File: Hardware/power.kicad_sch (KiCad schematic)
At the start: 52 parts, among them J1 USB4110GFA, Q1 AO3407A, U1 TPS54302, U2 USBLC6-2SC6, U3 INA226, U4 AP63205WU, U5 AP2112K-3.3, U6 AP7343-33W5-7

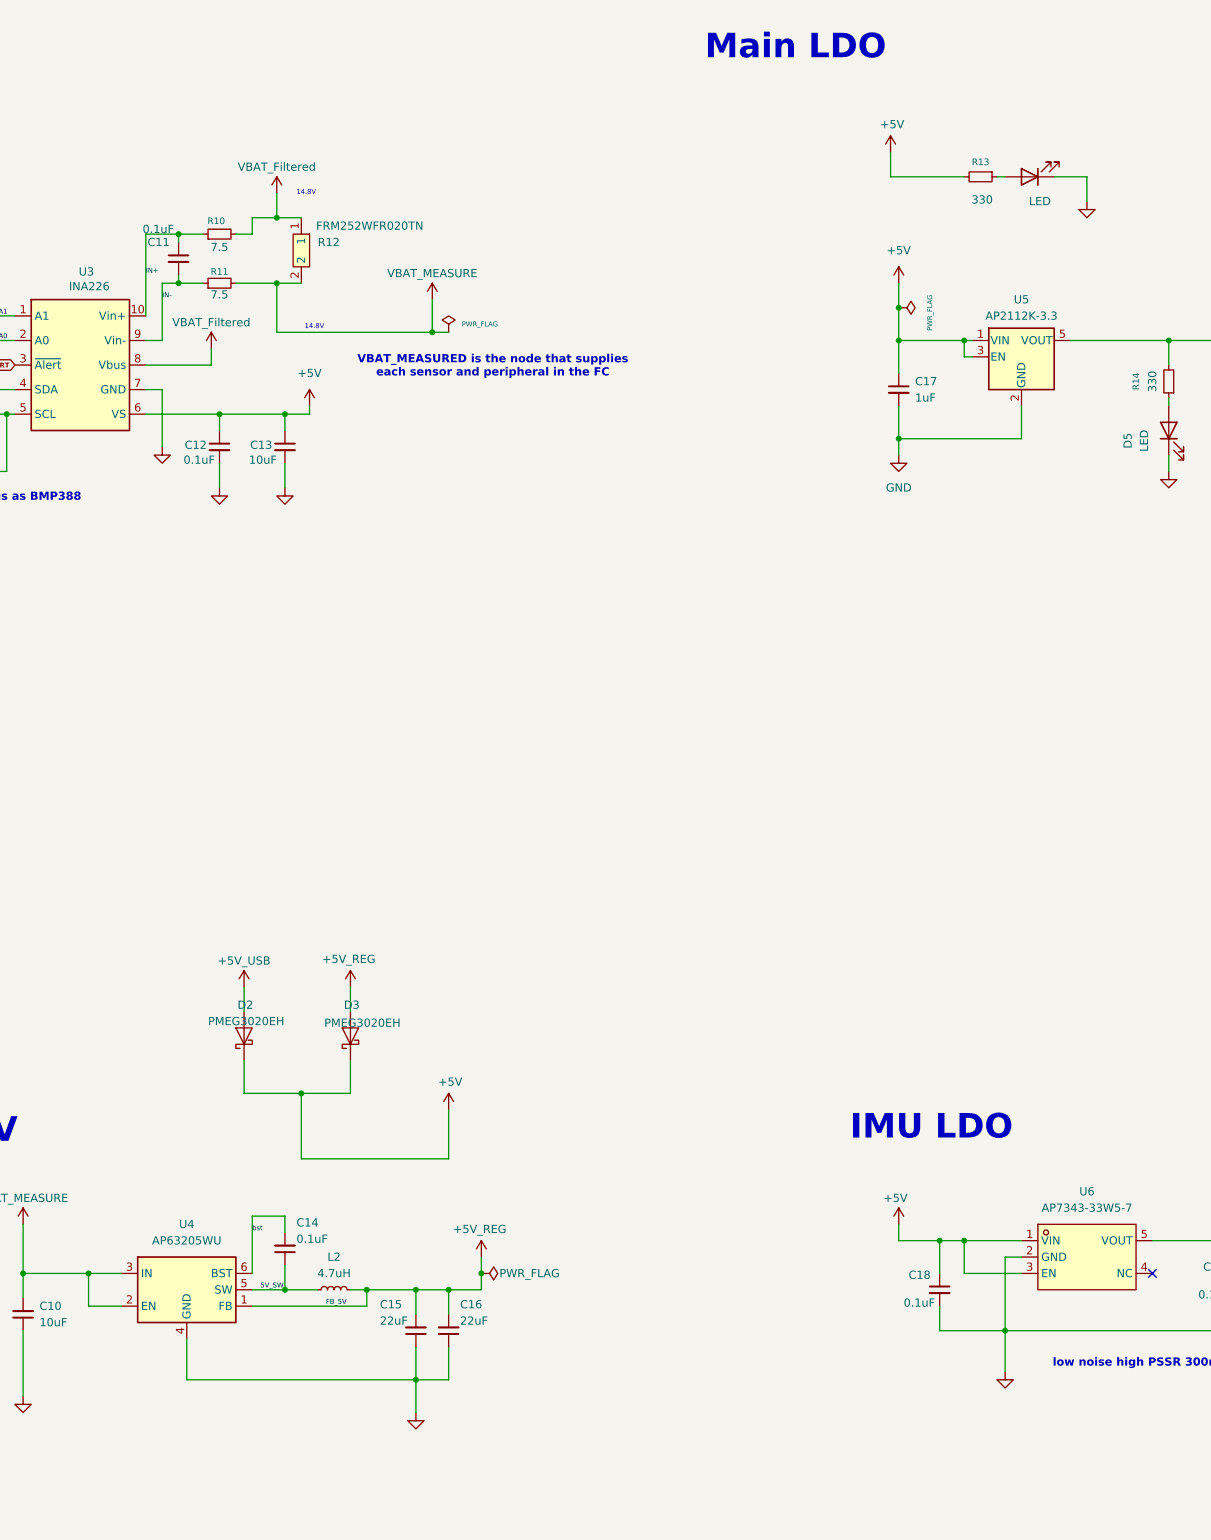
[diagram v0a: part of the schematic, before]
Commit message: progress layout
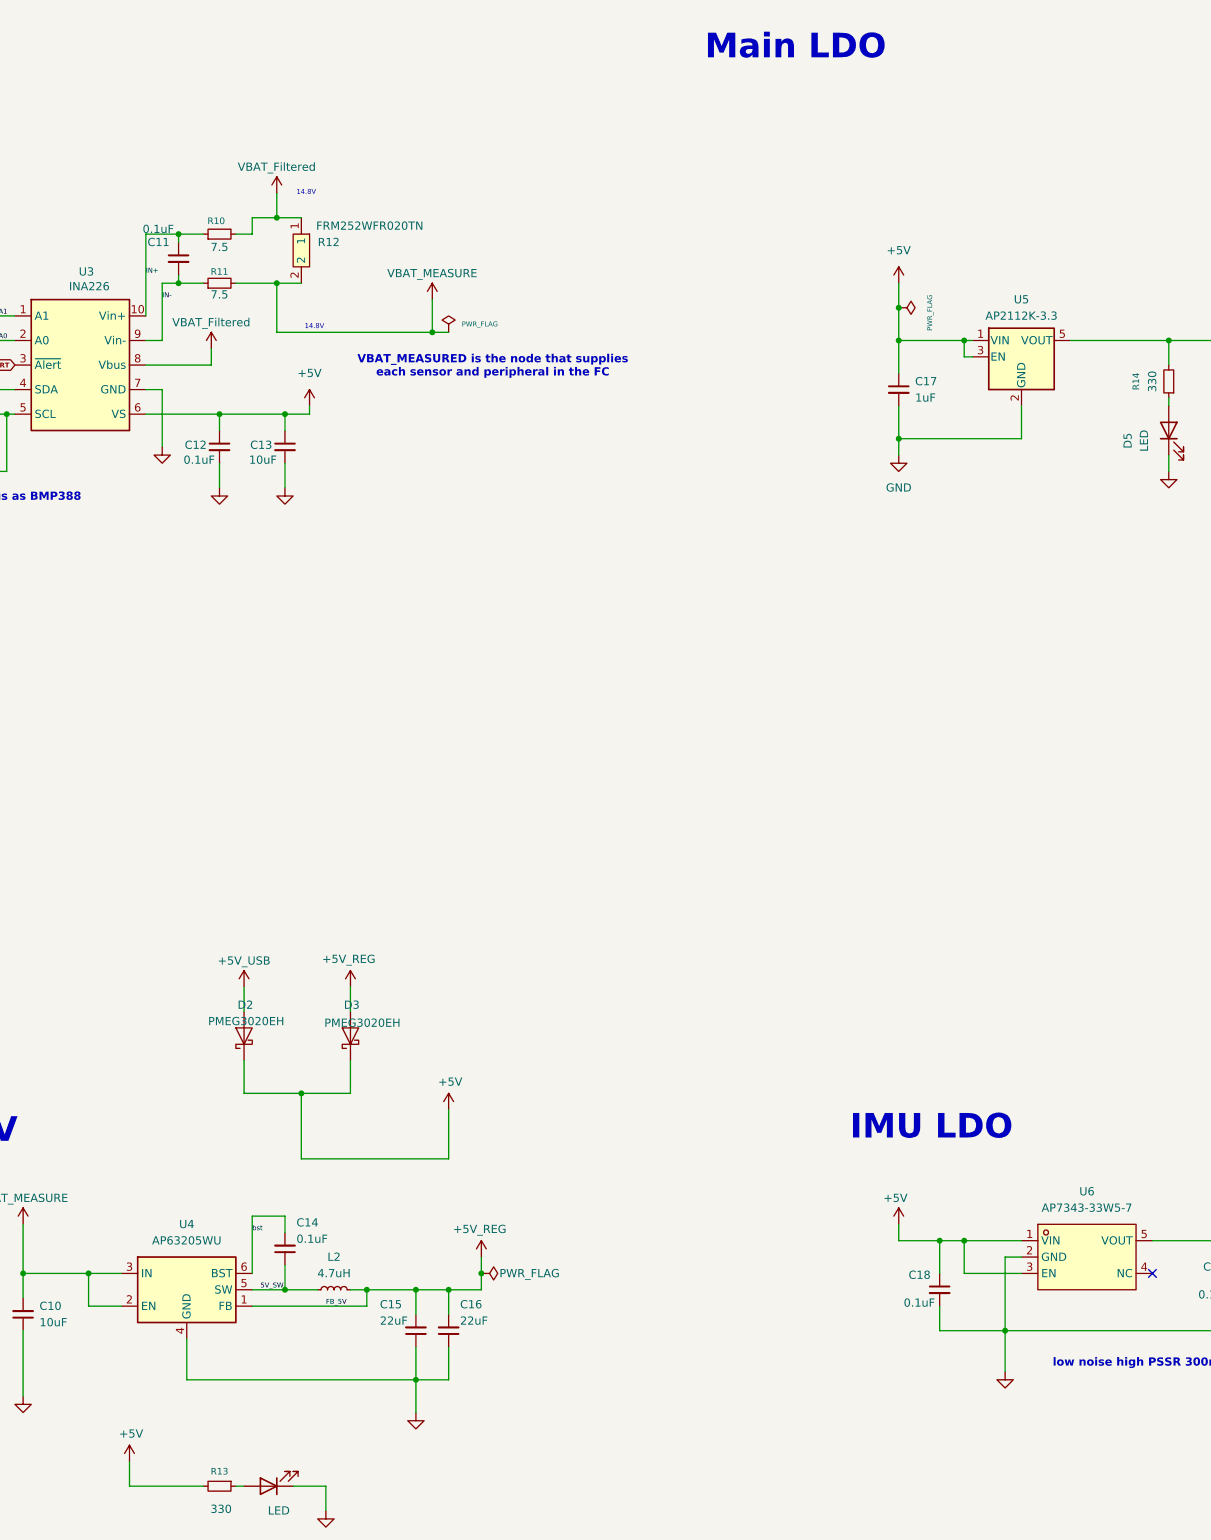
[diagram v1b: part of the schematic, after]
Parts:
- C2, C5: footprint Capacitor_SMD:C_0603_1608Metric -> Capacitor_SMD:C_0402_1005Metric
- D4: footprint LED_SMD:LED_0402_1005Metric -> LED_SMD:LED_0805_2012Metric
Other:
- moved on the sheet: R13
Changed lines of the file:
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@@
 	(wire
 		(pts
-			(xy 350.52 45.72) (xy 350.52 49.53)
+			(xy 232.41 248.92) (xy 232.41 252.73)
 		)
 		(stroke
@@
 	(wire
 		(pts
-			(xy 367.03 49.53) (xy 368.3 49.53)
+			(xy 248.92 252.73) (xy 250.19 252.73)
 		)
 		(stroke
@@
 	(wire
 		(pts
-			(xy 350.52 49.53) (xy 361.95 49.53)
+			(xy 232.41 252.73) (xy 243.84 252.73)
 		)
 		(stroke
@@
 	(wire
 		(pts
-			(xy 381 53.34) (xy 381 49.53)
+			(xy 262.89 256.54) (xy 262.89 252.73)
 		)
 		(stroke
@@
 	(wire
 		(pts
-			(xy 381 49.53) (xy 375.92 49.53)
+			(xy 262.89 252.73) (xy 257.81 252.73)
 		)
 		(stroke
@@
 	(symbol
 		(lib_id "power:GND")
-		(at 381 53.34 0)
+		(at 262.89 256.54 0)
 		(unit 1)
 		(exclude_from_sim no)
@@
 		(fields_autoplaced yes)
 		(property "Reference" "#PWR039"
-			(at 381 59.69 0)
+			(at 262.89 262.89 0)
 			(effects
 				(font
@@
 		)
 		(property "Value" "GND"
-			(at 381 58.42 0)
+			(at 262.89 261.62 0)
 			(effects
 				(font
@@
 		)
 		(property "Footprint" ""
-			(at 381 53.34 0)
+			(at 262.89 256.54 0)
 			(effects
 				(font
@@
 		)
 		(property "Datasheet" ""
-			(at 381 53.34 0)
+			(at 262.89 256.54 0)
 			(effects
 				(font
@@
 		)
 		(property "Description" "Power symbol creates a global label with name \"GND\" , ground"
-			(at 381 53.34 0)
+			(at 262.89 256.54 0)
 			(effects
 				(font
@@
 	(symbol
 		(lib_id "Device:R_Small")
-		(at 364.49 49.53 270)
+		(at 246.38 252.73 270)
 		(unit 1)
 		(exclude_from_sim no)
@@
 		(dnp no)
 		(property "Reference" "R13"
-			(at 364.49 47.244 90)
+			(at 246.38 250.444 90)
 			(effects
 				(font
@@
 		)
 		(property "Value" "330"
-			(at 364.744 53.086 90)
+			(at 246.634 256.286 90)
 			(effects
 				(font
@@
 		)
 		(property "Footprint" "Resistor_SMD:R_0402_1005Metric"
-			(at 364.49 49.53 0)
+			(at 246.38 252.73 0)
 			(effects
 				(font
@@
 		)
 		(property "Datasheet" "~"
-			(at 364.49 49.53 0)
+			(at 246.38 252.73 0)
 			(effects
 				(font
@@
 		)
 		(property "Description" "Resistor, small symbol"
-			(at 364.49 49.53 0)
+			(at 246.38 252.73 0)
 			(effects
 				(font
@@
 	(symbol
 		(lib_id "power:+5V")
-		(at 350.52 45.72 0)
+		(at 232.41 248.92 0)
 		(unit 1)
 		(exclude_from_sim no)
@@
 		(dnp no)
 		(property "Reference" "#PWR034"
-			(at 350.52 49.53 0)
+			(at 232.41 252.73 0)
 			(effects
 				(font
@@
 		)
 		(property "Value" "+5V"
-			(at 350.774 41.402 0)
+			(at 232.664 244.602 0)
 			(effects
 				(font
@@
 		)
 		(property "Footprint" ""
-			(at 350.52 45.72 0)
+			(at 232.41 248.92 0)
 			(effects
 				(font
@@
 		)
 		(property "Datasheet" ""
-			(at 350.52 45.72 0)
+			(at 232.41 248.92 0)
 			(effects
 				(font
@@
 		)
 		(property "Description" "Power symbol creates a global label with name \"+5V\""
-			(at 350.52 45.72 0)
+			(at 232.41 248.92 0)
 			(effects
 				(font
@@
 			)
 		)
-		(property "Footprint" "Capacitor_SMD:C_0603_1608Metric"
+		(property "Footprint" "Capacitor_SMD:C_0402_1005Metric"
 			(at 93.98 196.85 0)
 			(effects
@@
 	(symbol
 		(lib_id "Device:LED")
-		(at 372.11 49.53 180)
+		(at 254 252.73 180)
 		(unit 1)
 		(exclude_from_sim no)
@@
 		(dnp no)
 		(property "Reference" "D4"
-			(at 373.126 55.626 0)
+			(at 255.016 258.826 0)
 			(effects
 				(font
@@
 		)
 		(property "Value" "LED"
-			(at 373.6975 53.34 0)
+			(at 255.5875 256.54 0)
 			(effects
 				(font
@@
 			)
 		)
-		(property "Footprint" "LED_SMD:LED_0402_1005Metric"
-			(at 372.11 49.53 0)
+		(property "Footprint" "LED_SMD:LED_0805_2012Metric"
+			(at 254 252.73 0)
 			(effects
 				(font
@@
 		)
 		(property "Datasheet" "~"
-			(at 372.11 49.53 0)
+			(at 254 252.73 0)
 			(effects
 				(font
@@
 		)
 		(property "Description" "Light emitting diode"
-			(at 372.11 49.53 0)
+			(at 254 252.73 0)
 			(effects
 				(font
@@
 		)
 		(property "Sim.Pins" "1=K 2=A"
-			(at 372.11 49.53 0)
+			(at 254 252.73 0)
 			(effects
 				(font
@@
 			)
 		)
-		(property "Footprint" "Capacitor_SMD:C_0603_1608Metric"
+		(property "Footprint" "Capacitor_SMD:C_0402_1005Metric"
 			(at 52.07 200.66 0)
 			(effects
